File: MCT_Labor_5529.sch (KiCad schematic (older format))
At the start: 0 parts

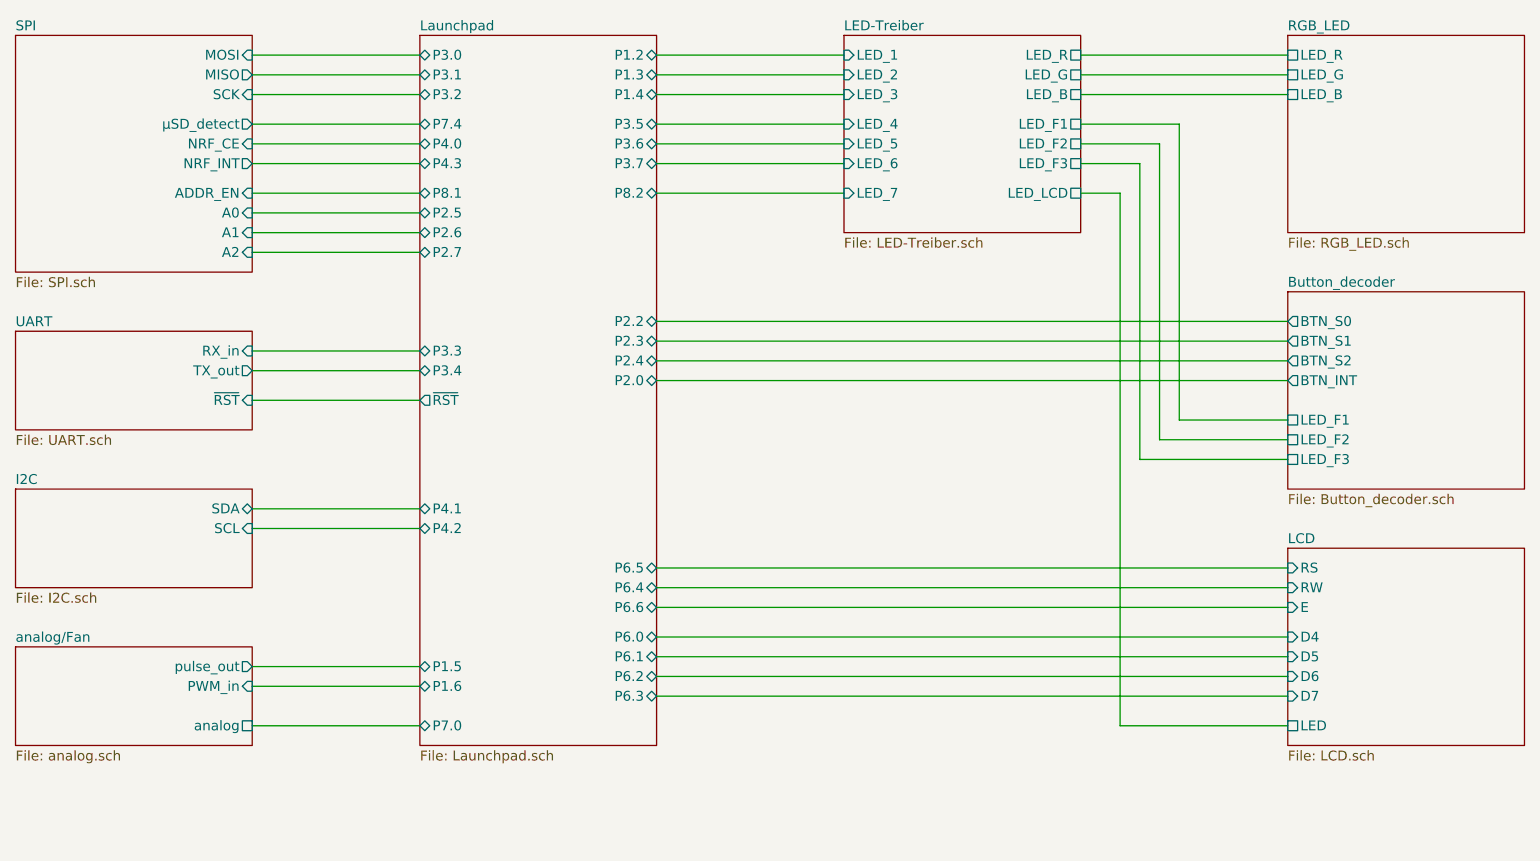
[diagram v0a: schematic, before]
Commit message: Erste fertige Version
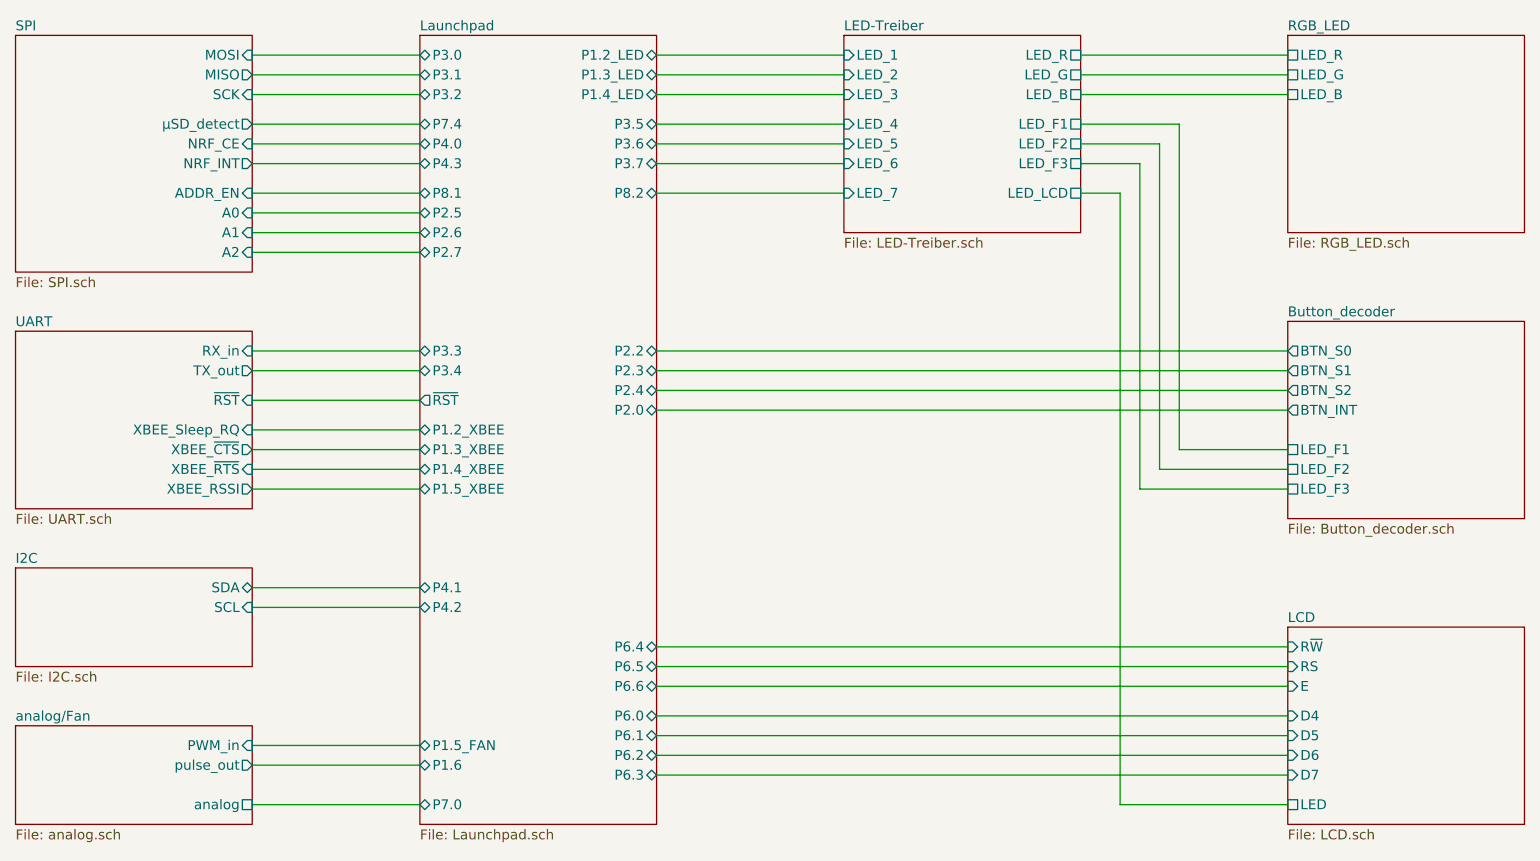
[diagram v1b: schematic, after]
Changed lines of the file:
@@
 $EndDescr
 $Sheet
-S 8750 4150 1200 1000
+S 8750 4550 1200 1000
 U 5EE928F9
 F0 "LCD" 50
 F1 "LCD.sch" 50
-F2 "D4" I L 8750 4600 50
-F3 "D5" I L 8750 4700 50
-F4 "D6" I L 8750 4800 50
-F5 "D7" I L 8750 4900 50
-F6 "RS" I L 8750 4250 50
-F7 "RW" I L 8750 4350 50
-F8 "E" I L 8750 4450 50
-F9 "LED" U L 8750 5050 50
-$EndSheet
-Wire Wire Line
-	8750 4900 5550 4900
+F2 "D4" I L 8750 5000 50
+F3 "D5" I L 8750 5100 50
+F4 "D6" I L 8750 5200 50
+F5 "D7" I L 8750 5300 50
+F6 "RS" I L 8750 4750 50
+F7 "R~W~" I L 8750 4650 50
+F8 "E" I L 8750 4850 50
+F9 "LED" U L 8750 5450 50
+$EndSheet
+Wire Wire Line
+	8750 5300 5550 5300
 $Sheet
 S 6500 1550 1200 1000
@@
 	7700 2350 7900 2350
 Wire Wire Line
-	7900 2350 7900 5050
-Wire Wire Line
-	7900 5050 8750 5050
+	7900 2350 7900 5450
+Wire Wire Line
+	7900 5450 8750 5450
 Wire Wire Line
 	6500 1650 5550 1650
@@
 	5550 2350 6500 2350
 $Sheet
-S 8750 2850 1200 1000
+S 8750 3000 1200 1000
 U 5EFA716B
 F0 "Button_decoder" 50
 F1 "Button_decoder.sch" 50
-F2 "BTN_S0" O L 8750 3000 50
-F3 "BTN_S1" O L 8750 3100 50
-F4 "BTN_S2" O L 8750 3200 50
-F5 "BTN_INT" O L 8750 3300 50
-F6 "LED_F1" U L 8750 3500 50
-F7 "LED_F2" U L 8750 3600 50
-F8 "LED_F3" U L 8750 3700 50
-$EndSheet
-Wire Wire Line
-	8200 2000 8200 3500
-Wire Wire Line
-	8200 3500 8750 3500
+F2 "BTN_S0" O L 8750 3150 50
+F3 "BTN_S1" O L 8750 3250 50
+F4 "BTN_S2" O L 8750 3350 50
+F5 "BTN_INT" O L 8750 3450 50
+F6 "LED_F1" U L 8750 3650 50
+F7 "LED_F2" U L 8750 3750 50
+F8 "LED_F3" U L 8750 3850 50
+$EndSheet
 Wire Wire Line
 	7700 2000 8200 2000
 Wire Wire Line
-	8750 3600 8100 3600
-Wire Wire Line
-	8100 3600 8100 2100
-Wire Wire Line
 	8100 2100 7700 2100
 Wire Wire Line
 	7700 2200 8000 2200
-Wire Wire Line
-	8000 2200 8000 3700
-Wire Wire Line
-	8000 3700 8750 3700
 $Sheet
 S 8750 1550 1200 1000
@@
 	7700 1850 8750 1850
 Wire Wire Line
-	5550 4800 8750 4800
-Wire Wire Line
-	5550 4700 8750 4700
-Wire Wire Line
-	5550 4600 8750 4600
-Wire Wire Line
-	5550 4450 8750 4450
-Wire Wire Line
-	5550 4350 8750 4350
-Wire Wire Line
-	5550 4250 8750 4250
-Wire Wire Line
-	5550 3300 8750 3300
-Wire Wire Line
-	5550 3200 8750 3200
-Wire Wire Line
-	5550 3100 8750 3100
-Wire Wire Line
-	5550 3000 8750 3000
-$Sheet
-S 4350 1550 1200 3600
-U 5F0B42CA
-F0 "Launchpad" 50
-F1 "Launchpad.sch" 50
-F2 "P6.5" B R 5550 4250 50
-F3 "P3.4" B L 4350 3250 50
-F4 "P3.3" B L 4350 3150 50
-F5 "P1.6" B L 4350 4850 50
-F6 "P6.6" B R 5550 4450 50
-F7 "P3.2" B L 4350 1850 50
-F8 "P2.7" B L 4350 2650 50
-F9 "P4.2" B L 4350 4050 50
-F10 "P4.1" B L 4350 3950 50
-F11 "P2.5" B L 4350 2450 50
-F12 "P2.4" B R 5550 3200 50
-F13 "P1.5" B L 4350 4750 50
-F14 "P1.4" B R 5550 1850 50
-F15 "P1.3" B R 5550 1750 50
-F16 "P1.2" B R 5550 1650 50
-F17 "P4.3" B L 4350 2200 50
-F18 "P4.0" B L 4350 2100 50
-F19 "P3.7" B R 5550 2200 50
-F20 "P8.2" B R 5550 2350 50
-F21 "P6.0" B R 5550 4600 50
-F22 "P6.1" B R 5550 4700 50
-F23 "P6.2" B R 5550 4800 50
-F24 "P6.3" B R 5550 4900 50
-F25 "P6.4" B R 5550 4350 50
-F26 "P7.0" B L 4350 5050 50
-F27 "P3.6" B R 5550 2100 50
-F28 "P3.5" B R 5550 2000 50
-F29 "P2.0" B R 5550 3300 50
-F30 "P2.2" B R 5550 3000 50
-F31 "P7.4" B L 4350 2000 50
-F32 "P3.0" B L 4350 1650 50
-F33 "P3.1" B L 4350 1750 50
-F34 "P2.6" B L 4350 2550 50
-F35 "P2.3" B R 5550 3100 50
-F36 "P8.1" B L 4350 2350 50
-F37 "~RST" O L 4350 3400 50
-$EndSheet
+	5550 5200 8750 5200
+Wire Wire Line
+	5550 5100 8750 5100
+Wire Wire Line
+	5550 5000 8750 5000
+Wire Wire Line
+	5550 4850 8750 4850
+Wire Wire Line
+	5550 4750 8750 4750
+Wire Wire Line
+	5550 4650 8750 4650
+Wire Wire Line
+	5550 3250 8750 3250
+Wire Wire Line
+	5550 3150 8750 3150
+Wire Wire Line
+	5550 3350 8750 3350
+Wire Wire Line
+	5550 3450 8750 3450
 $Sheet
 S 2300 1550 1200 1200
@@
 	3500 2650 4350 2650
 $Sheet
-S 2300 3050 1200 500
+S 2300 3050 1200 900
 U 5EFA875F
 F0 "UART" 50
@@
 F3 "TX_out" O R 3500 3250 50
 F4 "~RST" I R 3500 3400 50
-$EndSheet
-$Sheet
-S 2300 3850 1200 500
+F5 "XBEE_Sleep_RQ" I R 3500 3550 50
+F6 "XBEE_~CTS~" O R 3500 3650 50
+F7 "XBEE_~RTS~" I R 3500 3750 50
+F8 "XBEE_RSSI" O R 3500 3850 50
+$EndSheet
+$Sheet
+S 2300 4250 1200 500
 U 5EFA8860
 F0 "I2C" 50
 F1 "I2C.sch" 50
-F2 "SDA" B R 3500 3950 50
-F3 "SCL" I R 3500 4050 50
+F2 "SDA" B R 3500 4350 50
+F3 "SCL" I R 3500 4450 50
 $EndSheet
 Wire Wire Line
@@
 	4350 2000 3500 2000
 $Sheet
-S 2300 4650 1200 500
+S 2300 5050 1200 500
 U 5EFB1255
 F0 "analog/Fan" 50
 F1 "analog.sch" 50
-F2 "pulse_out" O R 3500 4750 50
-F3 "PWM_in" I R 3500 4850 50
-F4 "analog" U R 3500 5050 50
+F2 "pulse_out" O R 3500 5250 50
+F3 "PWM_in" I R 3500 5150 50
+F4 "analog" U R 3500 5450 50
 $EndSheet
 Wire Wire Line
@@
 	3500 3250 4350 3250
 Wire Wire Line
-	3500 3950 4350 3950
-Wire Wire Line
-	3500 4050 4350 4050
-Wire Wire Line
-	3500 5050 4350 5050
-Wire Wire Line
-	4350 4850 3500 4850
-Wire Wire Line
-	3500 4750 4350 4750
+	3500 4450 4350 4450
+$Sheet
+S 4350 1550 1200 4000
+U 5F0B42CA
+F0 "Launchpad" 50
+F1 "Launchpad.sch" 50
+F2 "P6.5" B R 5550 4750 50
+F3 "P3.4" B L 4350 3250 50
+F4 "P3.3" B L 4350 3150 50
+F5 "P1.6" B L 4350 5250 50
+F6 "P6.6" B R 5550 4850 50
+F7 "P3.2" B L 4350 1850 50
+F8 "P2.7" B L 4350 2650 50
+F9 "P4.2" B L 4350 4450 50
+F10 "P4.1" B L 4350 4350 50
+F11 "P2.5" B L 4350 2450 50
+F12 "P2.4" B R 5550 3350 50
+F13 "P4.3" B L 4350 2200 50
+F14 "P4.0" B L 4350 2100 50
+F15 "P3.7" B R 5550 2200 50
+F16 "P8.2" B R 5550 2350 50
+F17 "P6.0" B R 5550 5000 50
+F18 "P6.1" B R 5550 5100 50
+F19 "P6.2" B R 5550 5200 50
+F20 "P6.3" B R 5550 5300 50
+F21 "P6.4" B R 5550 4650 50
+F22 "P7.0" B L 4350 5450 50
+F23 "P3.6" B R 5550 2100 50
+F24 "P3.5" B R 5550 2000 50
+F25 "P2.0" B R 5550 3450 50
+F26 "P2.2" B R 5550 3150 50
+F27 "P7.4" B L 4350 2000 50
+F28 "P3.0" B L 4350 1650 50
+F29 "P3.1" B L 4350 1750 50
+F30 "P2.6" B L 4350 2550 50
+F31 "P2.3" B R 5550 3250 50
+F32 "P8.1" B L 4350 2350 50
+F33 "~RST" O L 4350 3400 50
+F34 "P1.4_LED" B R 5550 1850 50
+F35 "P1.3_LED" B R 5550 1750 50
+F36 "P1.2_LED" B R 5550 1650 50
+F37 "P1.2_XBEE" B L 4350 3550 50
+F38 "P1.3_XBEE" B L 4350 3650 50
+F39 "P1.4_XBEE" B L 4350 3750 50
+F40 "P1.5_FAN" B L 4350 5150 50
+F41 "P1.5_XBEE" B L 4350 3850 50
+$EndSheet
+Wire Wire Line
+	3500 3550 4350 3550
+Wire Wire Line
+	4350 3650 3500 3650
+Wire Wire Line
+	3500 3750 4350 3750
+Wire Wire Line
+	3500 5450 4350 5450
+Wire Wire Line
+	4350 5150 3500 5150
+Wire Wire Line
+	3500 4350 4350 4350
+Wire Wire Line
+	3500 5250 4350 5250
+Wire Wire Line
+	3500 3850 4350 3850
+Wire Wire Line
+	8000 3850 8750 3850
+Wire Wire Line
+	8000 2200 8000 3850
+Wire Wire Line
+	8750 3750 8100 3750
+Wire Wire Line
+	8100 2100 8100 3750
+Wire Wire Line
+	8200 3650 8750 3650
+Wire Wire Line
+	8200 2000 8200 3650
 $EndSCHEMATC
